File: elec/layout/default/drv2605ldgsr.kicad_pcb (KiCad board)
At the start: 2 copper layers, 225.7 x 100.8 mm, 0 parts

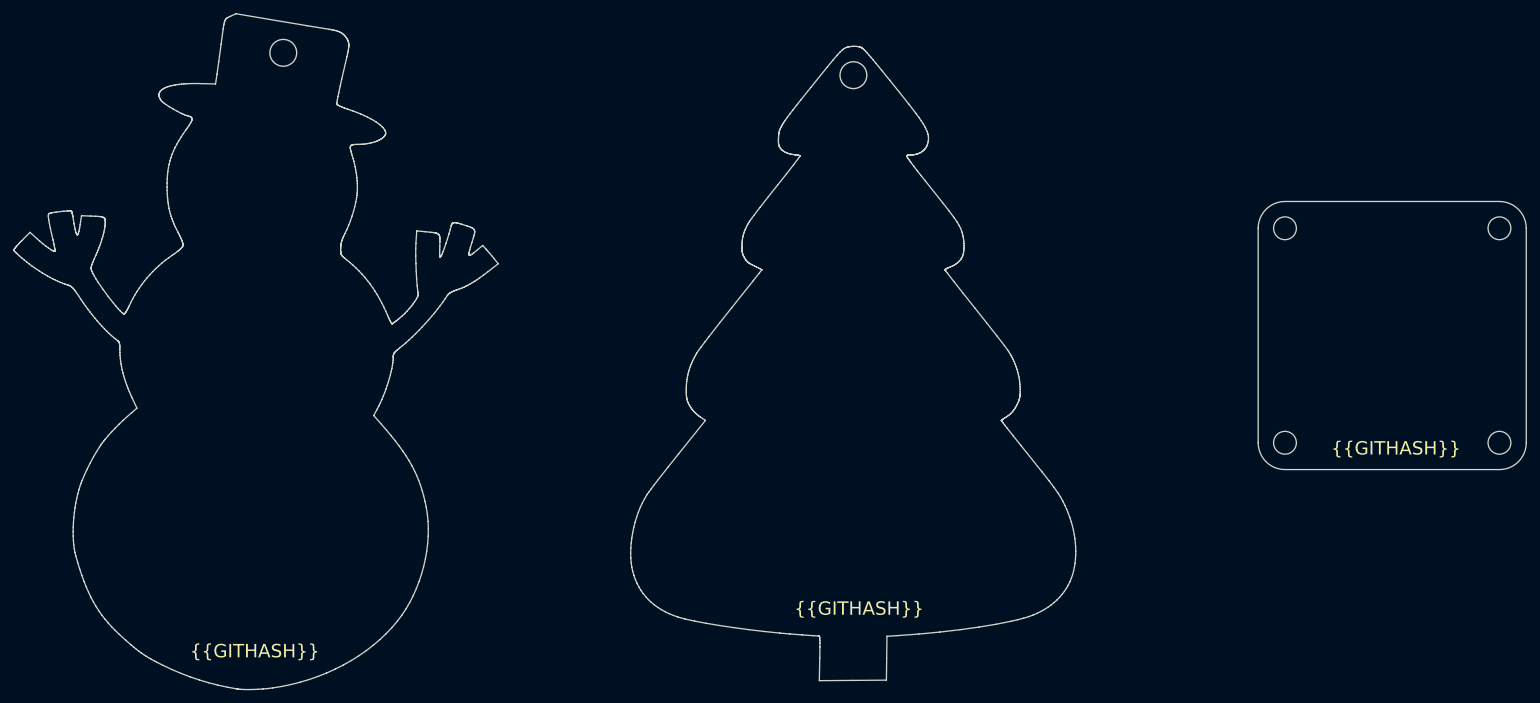
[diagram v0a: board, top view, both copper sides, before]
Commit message: layout
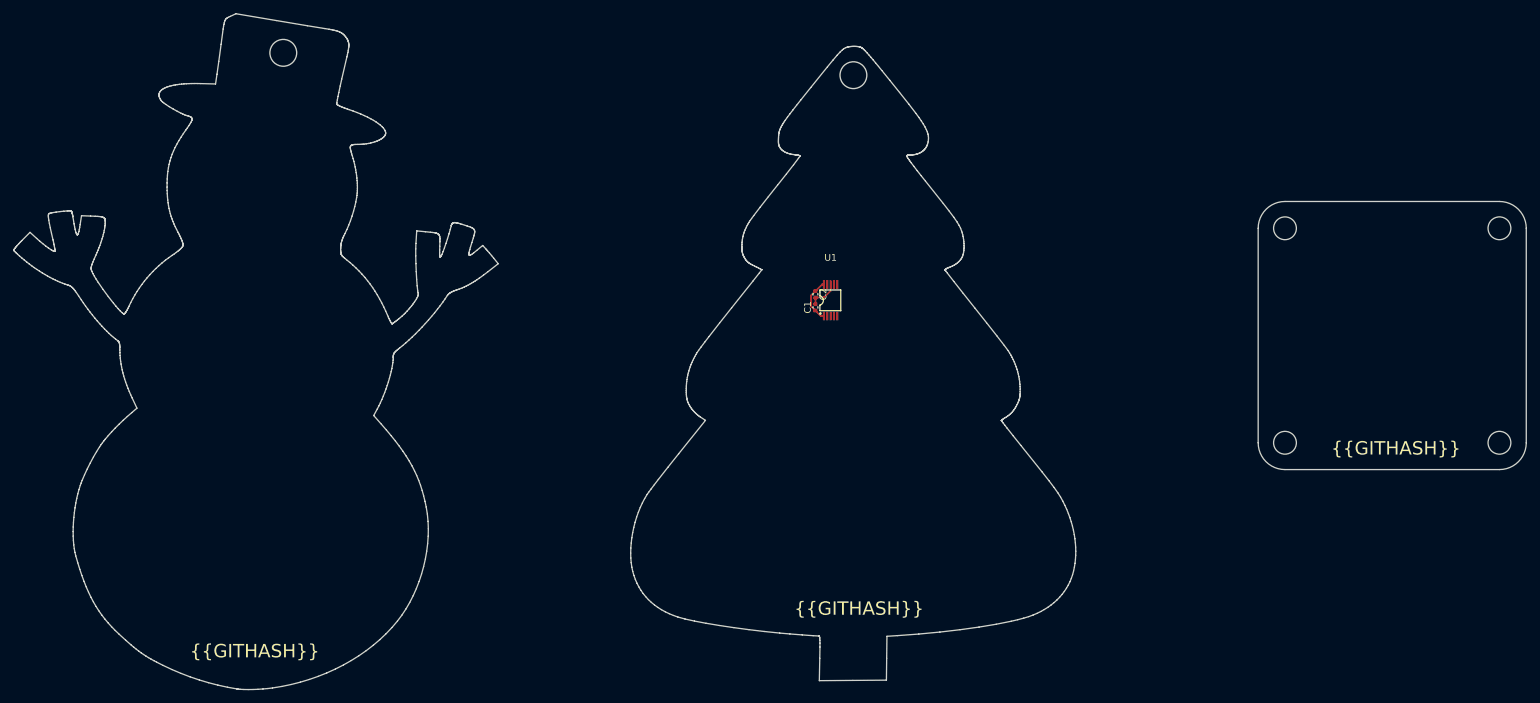
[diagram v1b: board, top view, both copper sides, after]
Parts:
- added C1: Multilayer Ceramic Capacitors MLCC - SMD/SMT 1uF 6.3V 0402 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, lib:C0402, F.Cu at (155.6, 93.6)
- added C2: Multilayer Ceramic Capacitors MLCC - SMD/SMT 1uF 6.3V 0402 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, lib:C0402, F.Cu at (155.6, 91.6)
- added U1: , lib:VSSOP-10_L3.0-W3.0-P0.50-LS4.9-BL, F.Cu at (157.8, 92.5)
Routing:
- net vcc: track 0.00 -> 6.71 mm
- net gnd: track 0.00 -> 4.62 mm
